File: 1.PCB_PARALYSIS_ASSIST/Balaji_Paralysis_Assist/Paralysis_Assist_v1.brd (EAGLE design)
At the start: 106.7 x 100 mm, 24 parts, among them IC2 7805TV, U1 ZC563900

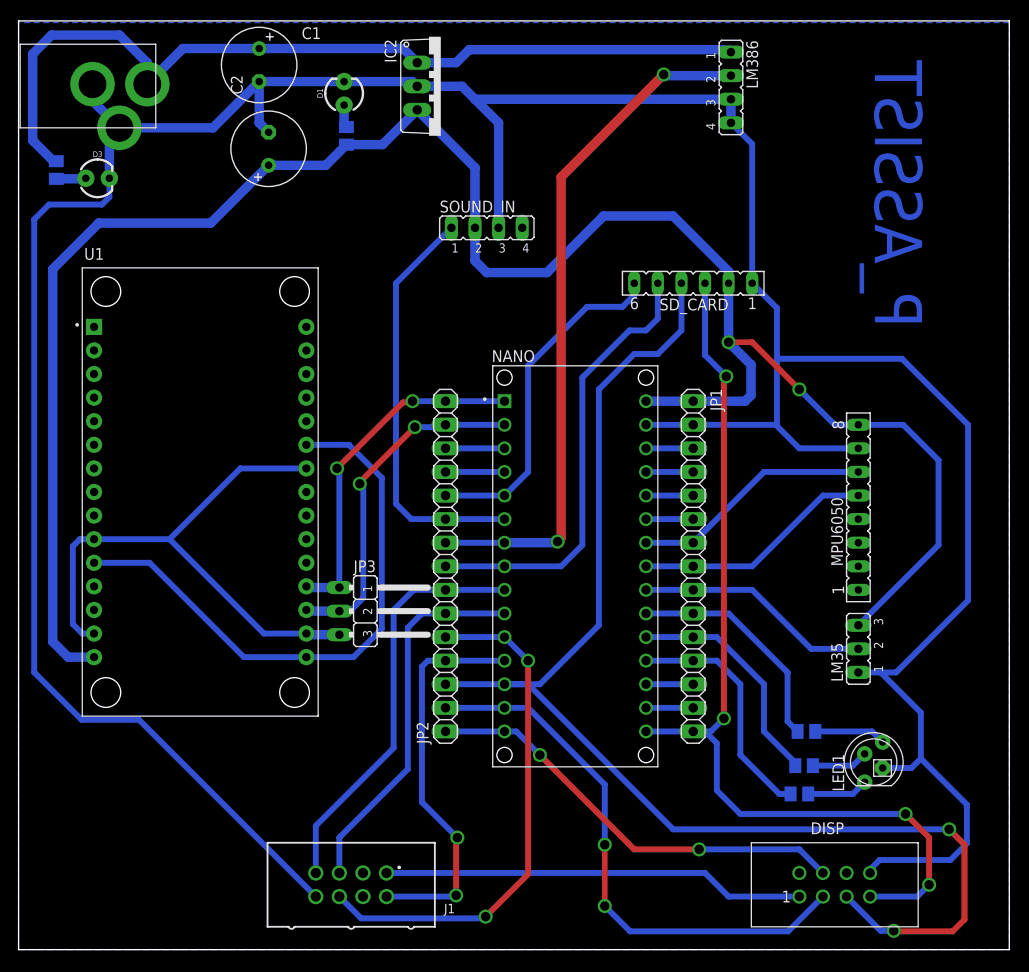
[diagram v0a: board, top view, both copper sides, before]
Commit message: added image
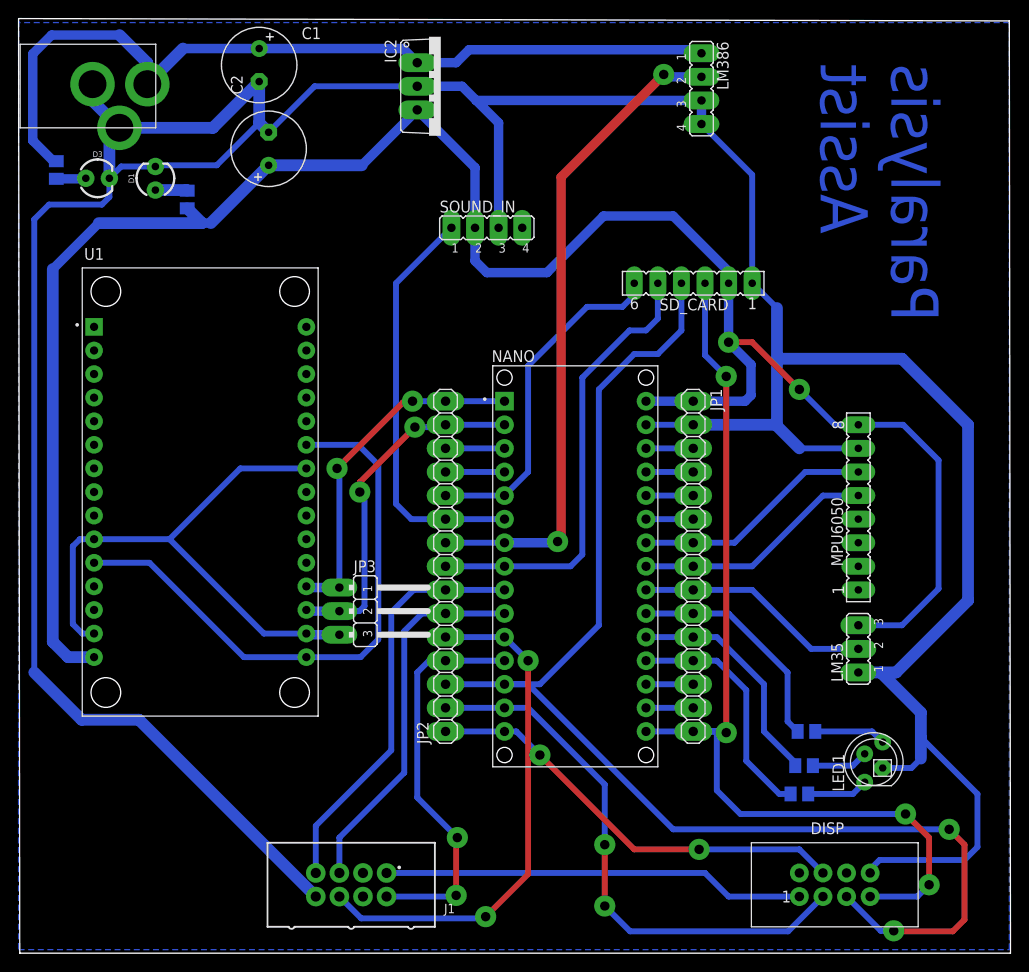
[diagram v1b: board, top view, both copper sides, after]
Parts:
- moved D1 22.3 mm to (14.7, 83.1)
- moved R1 18.5 mm to (18.2, 80.8)
- moved LM386 3.18 mm to (73.5, 92.7)
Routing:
- net GND: track 360.0 -> 381.4 mm
- net 5V: track 218.6 -> 223.6 mm
- net AUDIO_OUT: track 74.4 -> 71.3 mm
- net 9_IN: track 95.2 -> 92.1 mm
- net SCK: track 101.9 -> 103.8 mm
- net N$3: track 2.46 -> 3.46 mm
- net 3V3: track 62.3 -> 63.0 mm
- net RXNANO: track 37.5 -> 38.2 mm
- net MISO: track 48.3 -> 48.9 mm
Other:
- board size 106.7 x 100 mm -> 106.8 x 100.6 mm
- board text added: "Paralysis Assist"
- board text removed: "P_ASSIST"
